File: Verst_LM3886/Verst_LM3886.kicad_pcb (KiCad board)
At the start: 2 copper layers, 72 x 63.5 mm, 29 parts, among them J1 AudioJack3_Ground, J2 Conn_01x02_Pin, J3 Conn_01x05_Pin, U1 LM3886

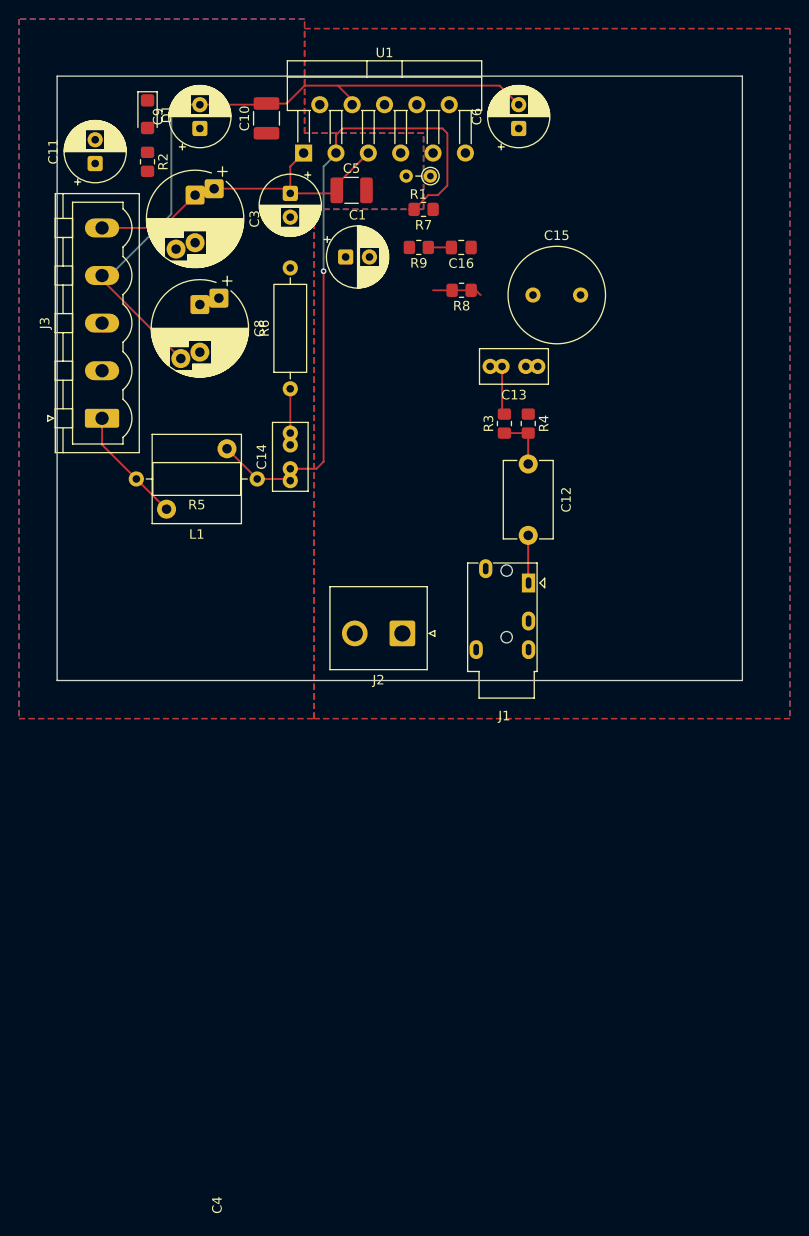
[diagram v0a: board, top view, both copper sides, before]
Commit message: Erste Testversion der Platine abgeschlossen
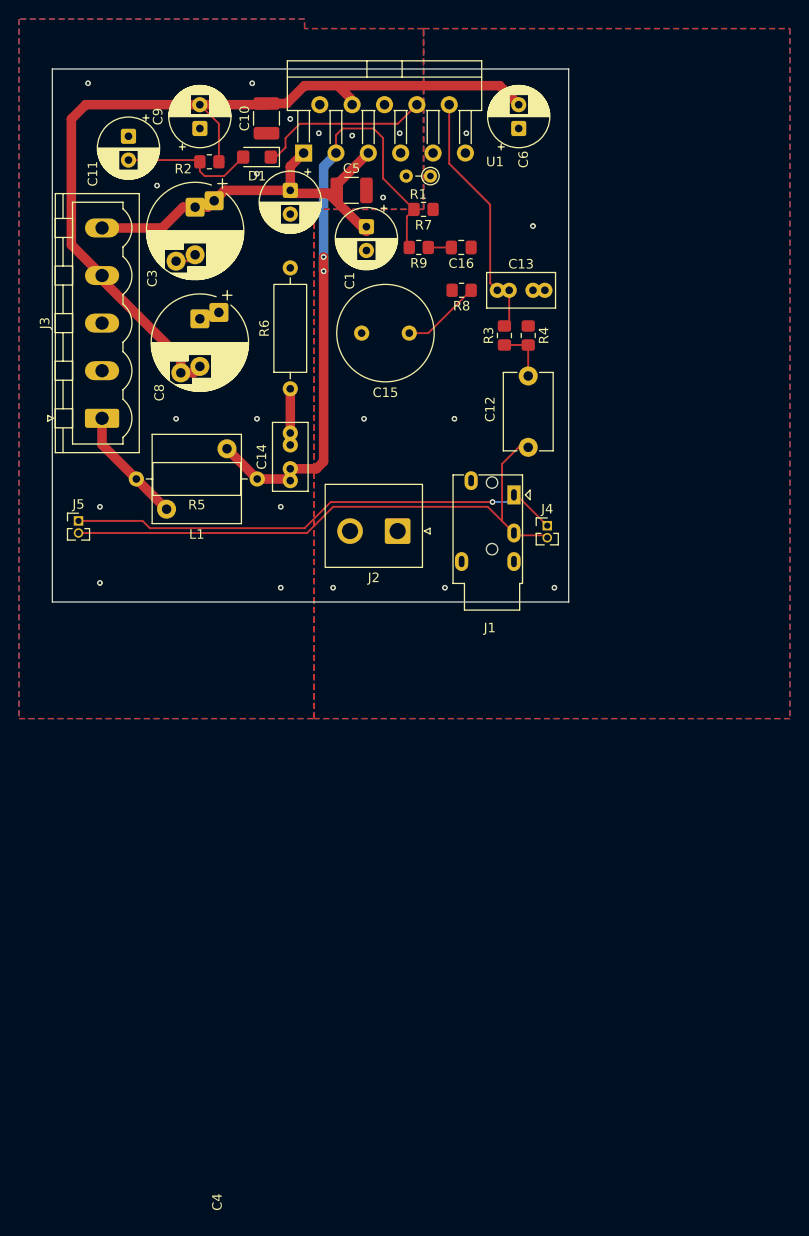
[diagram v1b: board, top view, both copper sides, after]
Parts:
- added J4: Conn_01x02_Pin, Connector_PinHeader_1.27mm:PinHeader_1x02_P1.27mm_Vertical, F.Cu at (234.0, 119.7)
- added J5: Conn_01x02_Pin, Connector_PinHeader_1.27mm:PinHeader_1x02_P1.27mm_Vertical, F.Cu at (184.8, 119.2)
- moved C15 13.6 mm to (219.5, 99.5), turned to 180 degrees
- moved D1 12.3 mm to (203.5, 81.0), turned to 180 degrees
- moved J2 10.8 mm to (218.3, 120.3)
- moved J1 9.38 mm to (230.5, 116.5)
- moved C12 9.25 mm to (232.0, 104.0)
- moved R3 9.25 mm to (229.5, 99.8)
- moved R4 9.25 mm to (232.0, 99.8)
- moved C13 8.04 mm to (233.8, 95.0)
- moved R2 6.50 mm to (198.5, 81.5), turned to 0 degrees
- moved C11 4.52 mm to (190.0, 78.8), turned to -90 degrees
- moved C1 3.86 mm to (215.0, 88.3), turned to -90 degrees
- moved C8 1.50 mm to (197.5, 98.0)
- moved C3 1.27 mm to (197.0, 86.3)
- moved C4 0.32 mm to (207.0, 84.5)
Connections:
- C12 pad 2: Net-(C12-Pad2) -> Net-(J4-Pin_2)
- J1 pad T: Net-(C12-Pad2) -> Net-(J4-Pin_1)
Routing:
- net Net-(J4-Pin_2): track 0.00 -> 61.2 mm
- net Net-(J4-Pin_1): track 0.00 -> 52.4 mm, vias 0 -> 1
- net Net-(U1-+): track 5.10 -> 25.5 mm
- net -24V: track 74.1 -> 93.1 mm
- net Net-(D1-K): track 0.00 -> 18.2 mm
- net Net-(D1-A): track 0.00 -> 14.2 mm
- net +24V: track 34.5 -> 43.9 mm
- net Net-(C12-Pad2): track 5.01 -> 0.00 mm
- net Net-(C15-Pad1): track 5.21 -> 8.36 mm
- net GND: track 0.00 -> 2.28 mm, vias 0 -> 15
- net Net-(C14-Pad1): track 69.4 -> 67.6 mm, vias 1 -> 2
- net GNDS: vias 0 -> 7
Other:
- board size 72 x 63.5 mm -> 54.2 x 56 mm
